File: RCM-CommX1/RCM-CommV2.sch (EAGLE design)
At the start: 25 parts, among them J1 BLACKFIN_HEADER, J2- C-GRID-04

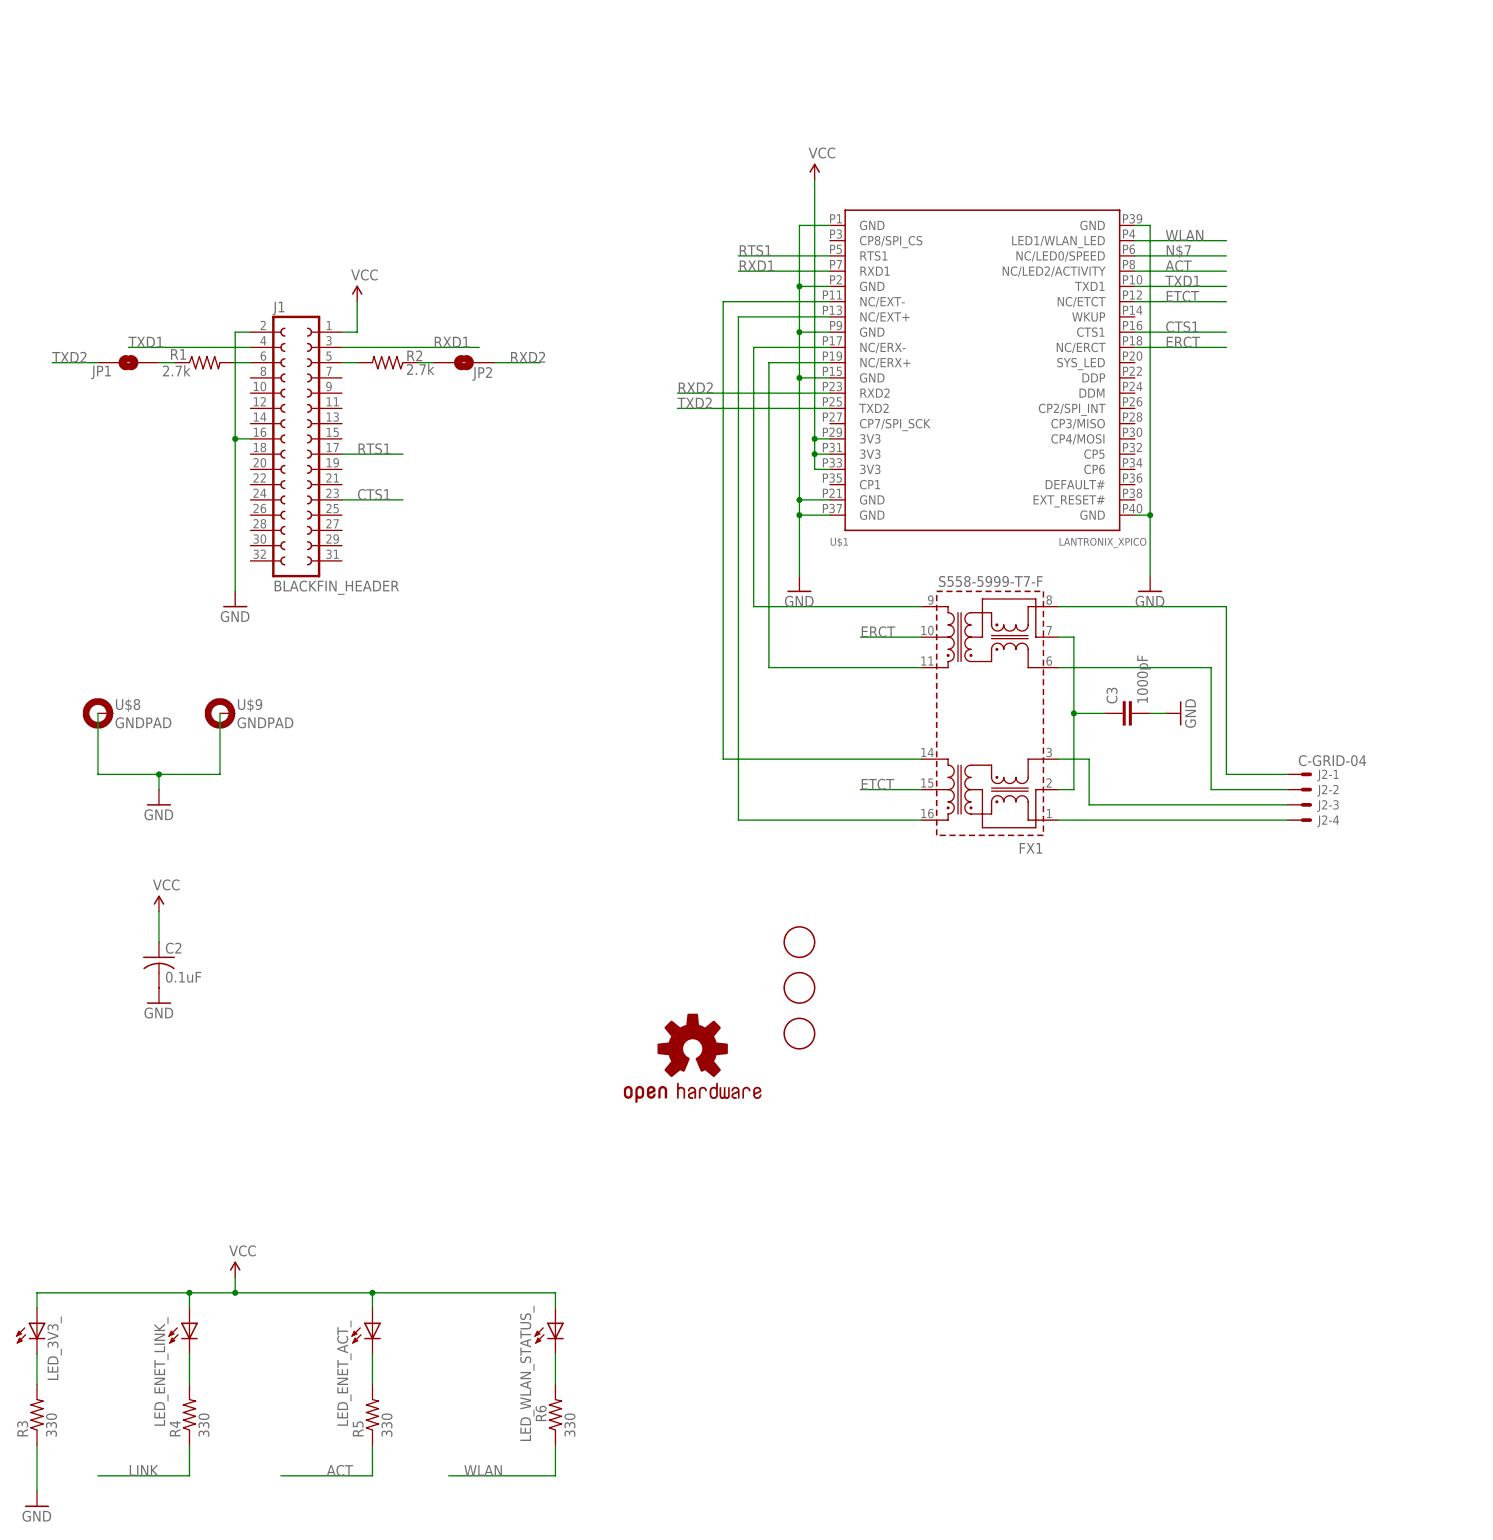
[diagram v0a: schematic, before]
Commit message: Version 2.0 of RCM-Comm board ready for review.
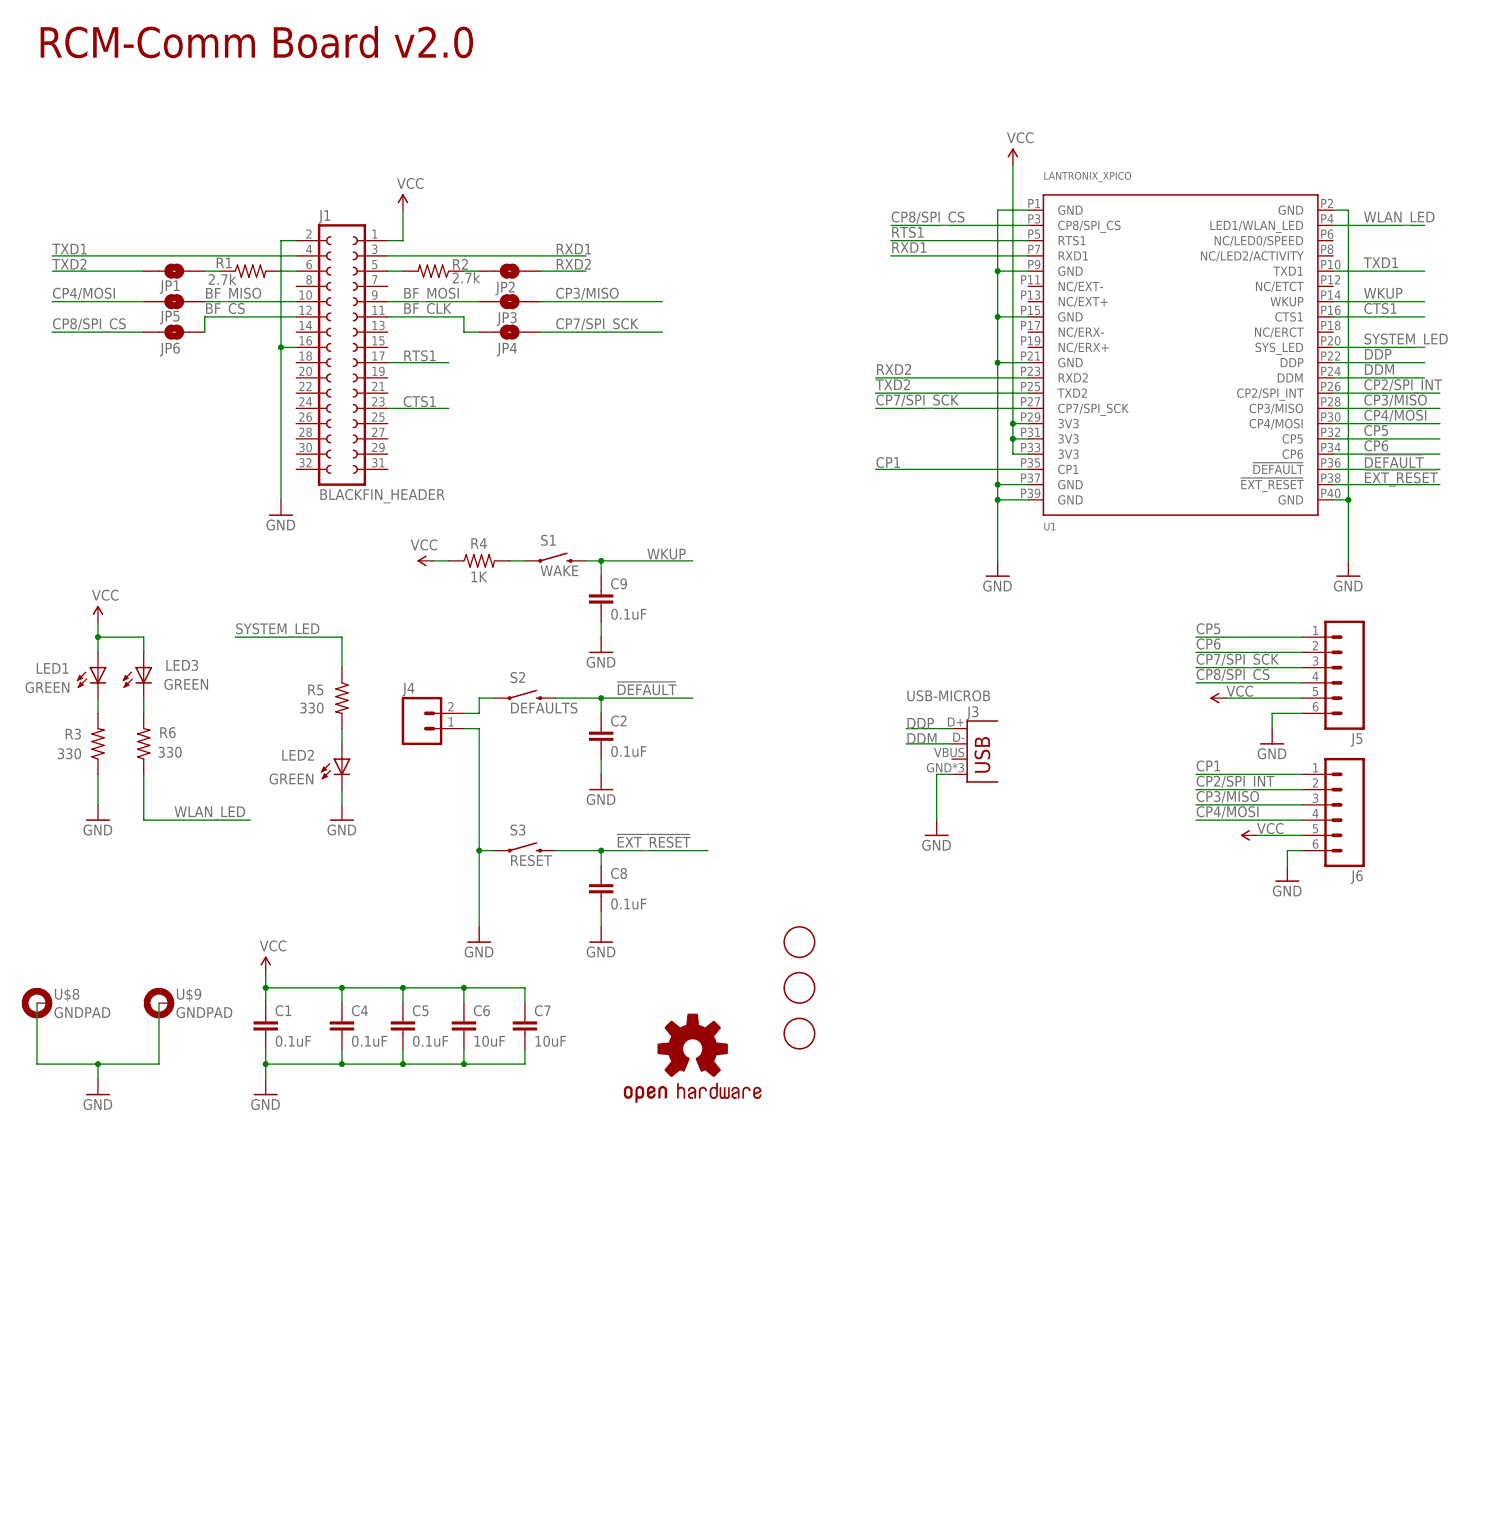
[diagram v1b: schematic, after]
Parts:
- removed C3: 1000pF, spark_fun:CAP0603-CAP
- removed FX1: S558-5999-T7-F, halo-electronics:TG110-E050N5
- removed J2-: C-GRID-04, MolexConnector:C-GRID-04
- removed LED_3V3_, LED_ENET_ACT_, LED_ENET_LINK_, LED_WLAN_STATUS_: (no value), spark_fun:LED0603
- removed U$1: LANTRONIX_XPICO, xPico:LANTRONIX_XPICO
- added C1, C4, C5, C8, C9: 0.1uF, SparkFun-Capacitors:0.1UF-25V(+80/-20%)(0603)
- added C6, C7: 10uF, SparkFun-Capacitors:10UF-6.3V-20%(0603)
- added J3: USB-MICROB, SparkFun-Connectors:USB-MICROB
- added J4: (no value), SparkFun-Connectors:M02LOCK
- added J5, J6: (no value), SparkFun-Connectors:M06LOCK
- added JP3, JP4, JP5, JP6: JUMPER-PAD-2-NOROUND, SparkFun-Passives:JUMPER-PAD-2-NOROUND
- added LED1, LED2, LED3: GREEN, spark_fun:LED0603
- added S1: WAKE, SparkFun-Electromechanical:SWITCH-MOMENTARY-2SMD
- added S2: DEFAULTS, SparkFun-Electromechanical:SWITCH-MOMENTARY-2SMD
- added S3: RESET, SparkFun-Electromechanical:SWITCH-MOMENTARY-2SMD
- added U1: LANTRONIX_XPICO, xPico:LANTRONIX_XPICO
- C2: device rcl:C-USC0603 -> SparkFun-Capacitors:0.1UF-25V(+80/-20%)(0603)
- R4: value 330 -> 1K; device spark_fun:RESISTOR0603-RES -> rcl:R-US_R0603
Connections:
- removed net ACT: R5.1, U$1.NC/LED2/ACTIVITY
- removed net ERCT: FX1.10, U$1.NC/ERCT
- removed net ETCT: FX1.15, U$1.NC/ETCT
- removed net LINK: R4.1
- removed net N$13: FX1.16, U$1.NC/EXT+
- removed net N$14: FX1.14, U$1.NC/EXT-
- removed net N$16: FX1.11, U$1.NC/ERX+
- removed net N$17: FX1.9, U$1.NC/ERX-
- removed net N$18: FX1.1, J2-4.S
- removed net N$19: FX1.3, J2-3.S
- removed net N$20: FX1.8, J2-1.S
- removed net N$21: FX1.6, J2-2.S
- removed net N$7: U$1.NC/LED0/SPEED
- removed net WLAN: R6.1, U$1.LED1/WLAN_LED
- new net !DEFAULT!: C2.1, S2.2, U1.!DEFAULT!
- new net !EXT_RESET!: C8.1, S3.2, U1.!EXT_RESET!
- new net BF_CLK: J1.SPI_SCK, JP4.1
- new net BF_CS: J1.SPI_SEL, JP6.2
- new net BF_MISO: J1.SPI_MISO, JP5.2
- new net BF_MOSI: J1.SPI_MOSI, JP3.1
- new net CP1: J6.1, U1.CP1
- new net CP2/SPI_INT: J6.2, U1.CP2/SPI_INT
- new net CP3/MISO: J6.3, JP3.2, U1.CP3/MISO
- new net CP4/MOSI: J6.4, JP5.1, U1.CP4/MOSI
- new net CP5: J5.1, U1.CP5
- new net CP6: J5.2, U1.CP6
- new net CP7/SPI_SCK: J5.3, JP4.2, U1.CP7/SPI_SCK
- new net CP8/SPI_CS: J5.4, JP6.1, U1.CP8/SPI_CS
- new net DDM: J3.D-, U1.DDM
- new net DDP: J3.D+, U1.DDP
- new net SYSTEM_LED: R5.1, U1.SYS_LED
- new net WKUP: C9.1, S1.2, U1.WKUP
- new net WLAN_LED: R6.1, U1.LED1/WLAN_LED
- net CTS1: now also U1.CTS1; no longer U$1.CTS1
- net GND: now also C1.2, C4.2, C5.2, C6.2, C7.2, C8.2, C9.2, J3.GND, J4.1, J5.6, J6.6, LED2.C, S3.1, U1.GND@1, U1.GND@2, U1.GND@3, U1.GND@4, U1.GND@5, U1.GND@6, U1.GND@7, U1.GND@8; no longer C3.2, U$1.GND@1, U$1.GND@2, U$1.GND@3, U$1.GND@4, U$1.GND@5, U$1.GND@6, U$1.GND@7, U$1.GND@8
- net N$1: now also J4.2, S2.1; no longer C3.1, FX1.2, FX1.7
- net N$3: now also LED1.C; no longer LED_3V3_.C
- net N$5: now also S1.1; no longer LED_ENET_LINK_.C
- net N$6: now also LED2.A; no longer LED_ENET_ACT_.C
- net N$8: now also LED3.C; no longer LED_WLAN_STATUS_.C
- net RTS1: now also U1.RTS1; no longer U$1.RTS1
- net RXD1: now also U1.RXD1; no longer U$1.RXD1
- net RXD2: now also U1.RXD2; no longer U$1.RXD2
- net TXD1: now also U1.TXD1; no longer U$1.TXD1
- net TXD2: now also U1.TXD2; no longer U$1.TXD2
- net VCC: now also C1.1, C4.1, C5.1, C6.1, C7.1, J5.5, J6.5, LED1.A, LED3.A, R4.1, U1.3V3@1, U1.3V3@2, U1.3V3@3; no longer C2.1, LED_3V3_.A, LED_ENET_ACT_.A, LED_ENET_LINK_.A, LED_WLAN_STATUS_.A, U$1.3V3@1, U$1.3V3@2, U$1.3V3@3
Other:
- note added: "Do Not Place"
- note added: "RCM-Comm Board v2.0"
- moved on the sheet: C2, J1, JP1, JP2, R1, R2, R3, R4, R5, R6, U$8, U$9
